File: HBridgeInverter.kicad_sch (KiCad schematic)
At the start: 27 parts, among them Q1 NMOS, Q2 NMOS, Q3 NMOS, Q4 NMOS, Q5 NMOS, Q6 NMOS, Q7 NPN, U1 LM358

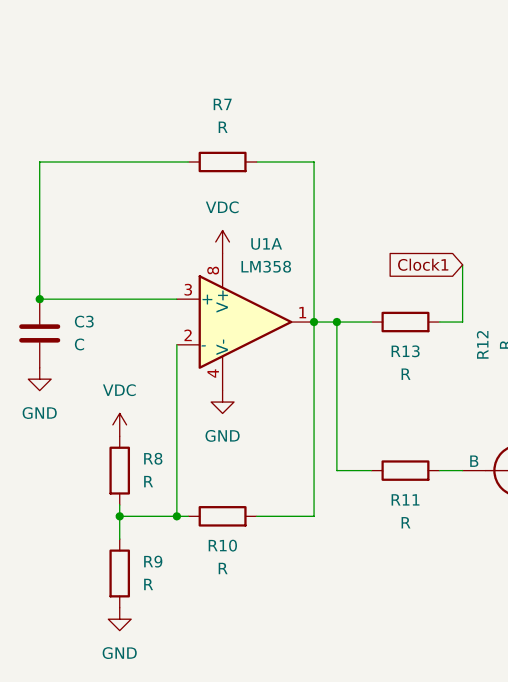
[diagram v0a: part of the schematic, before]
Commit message: whoops
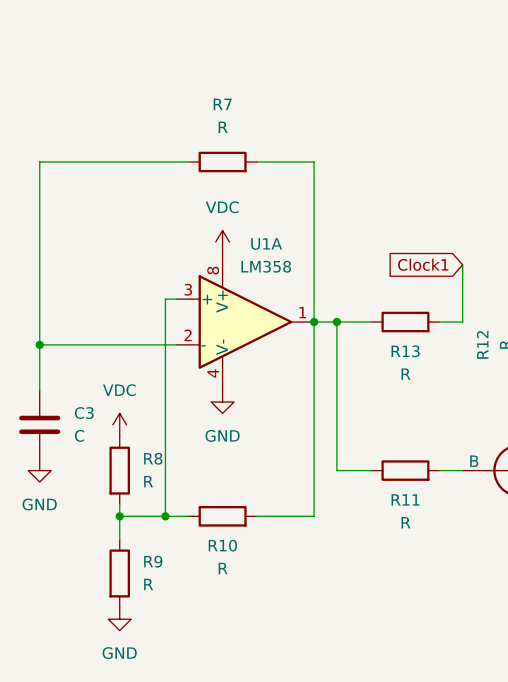
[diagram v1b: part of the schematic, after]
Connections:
- net at C3.1, R7.1: now also U1.2 (-); no longer U1.3 (+)
- net at R10.1, R8.2, R9.1: now also U1.3 (+); no longer U1.2 (-)
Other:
- moved on the sheet: C3
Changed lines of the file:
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@@
+	)
+	(junction
+		(at 48.26 106.68)
+		(diameter 0)
+		(color 0 0 0 0)
 	)
 	(junction
@@
 	)
 	(junction
-		(at 67.31 85.09)
+		(at 34.29 87.63)
 		(diameter 0)
 		(color 0 0 0 0)
 	)
 	(junction
-		(at 34.29 82.55)
+		(at 67.31 85.09)
 		(diameter 0)
 		(color 0 0 0 0)
@@
 	)
 	(junction
-		(at 49.53 106.68)
-		(diameter 0)
-		(color 0 0 0 0)
-	)
-	(junction
 		(at 190.5 81.28)
 		(diameter 0)
@@
 	(wire
 		(pts
+			(xy 48.26 106.68) (xy 50.8 106.68)
+		)
+		(stroke
+			(width 0)
+			(type default)
+		)
+	)
+	(wire
+		(pts
 			(xy 203.2 57.15) (xy 215.9 57.15)
 		)
@@
 	(wire
 		(pts
-			(xy 49.53 106.68) (xy 50.8 106.68)
-		)
-		(stroke
-			(width 0)
-			(type default)
-		)
-	)
-	(wire
-		(pts
 			(xy 215.9 73.66) (xy 215.9 95.25)
 		)
@@
 	(wire
 		(pts
+			(xy 49.53 82.55) (xy 48.26 82.55)
+		)
+		(stroke
+			(width 0)
+			(type default)
+		)
+	)
+	(wire
+		(pts
 			(xy 190.5 81.28) (xy 203.2 81.28)
 		)
@@
 	(wire
 		(pts
+			(xy 34.29 87.63) (xy 49.53 87.63)
+		)
+		(stroke
+			(width 0)
+			(type default)
+		)
+	)
+	(wire
+		(pts
 			(xy 64.77 67.31) (xy 64.77 85.09)
 		)
@@
 	(wire
 		(pts
+			(xy 34.29 87.63) (xy 34.29 92.71)
+		)
+		(stroke
+			(width 0)
+			(type default)
+		)
+	)
+	(wire
+		(pts
 			(xy 78.74 101.6) (xy 81.28 101.6)
 		)
@@
 	(wire
 		(pts
-			(xy 49.53 87.63) (xy 49.53 106.68)
-		)
-		(stroke
-			(width 0)
-			(type default)
-		)
-	)
-	(wire
-		(pts
 			(xy 152.4 95.25) (xy 152.4 101.6)
 		)
@@
 	(wire
 		(pts
-			(xy 34.29 67.31) (xy 34.29 82.55)
+			(xy 34.29 67.31) (xy 34.29 87.63)
 		)
 		(stroke
@@
 	(wire
 		(pts
-			(xy 34.29 82.55) (xy 49.53 82.55)
-		)
-		(stroke
-			(width 0)
-			(type default)
-		)
-	)
-	(wire
-		(pts
-			(xy 43.18 106.68) (xy 49.53 106.68)
+			(xy 43.18 106.68) (xy 48.26 106.68)
 		)
 		(stroke
@@
 		(pts
 			(xy 58.42 106.68) (xy 64.77 106.68)
+		)
+		(stroke
+			(width 0)
+			(type default)
+		)
+	)
+	(wire
+		(pts
+			(xy 48.26 82.55) (xy 48.26 106.68)
 		)
 		(stroke
@@
 	(symbol
 		(lib_id "Device:C")
-		(at 34.29 86.36 0)
+		(at 34.29 96.52 0)
 		(unit 1)
 		(exclude_from_sim no)
@@
 		(fields_autoplaced yes)
 		(property "Reference" "C3"
-			(at 38.1 85.0899 0)
+			(at 38.1 95.2499 0)
 			(effects
 				(font
@@
 		)
 		(property "Value" "C"
-			(at 38.1 87.6299 0)
+			(at 38.1 97.7899 0)
 			(effects
 				(font
@@
 		)
 		(property "Footprint" ""
-			(at 35.2552 90.17 0)
+			(at 35.2552 100.33 0)
 			(effects
 				(font
@@
 		)
 		(property "Datasheet" "~"
-			(at 34.29 86.36 0)
+			(at 34.29 96.52 0)
 			(effects
 				(font
@@
 		)
 		(property "Description" "Unpolarized capacitor"
-			(at 34.29 86.36 0)
+			(at 34.29 96.52 0)
 			(effects
 				(font
@@
 	(symbol
 		(lib_id "power:GND")
-		(at 34.29 90.17 0)
+		(at 34.29 100.33 0)
 		(unit 1)
 		(exclude_from_sim no)
@@
 		(fields_autoplaced yes)
 		(property "Reference" "#PWR013"
-			(at 34.29 96.52 0)
+			(at 34.29 106.68 0)
 			(effects
 				(font
@@
 		)
 		(property "Value" "GND"
-			(at 34.29 95.25 0)
+			(at 34.29 105.41 0)
 			(effects
 				(font
@@
 		)
 		(property "Footprint" ""
-			(at 34.29 90.17 0)
+			(at 34.29 100.33 0)
 			(effects
 				(font
@@
 		)
 		(property "Datasheet" ""
-			(at 34.29 90.17 0)
+			(at 34.29 100.33 0)
 			(effects
 				(font
@@
 		)
 		(property "Description" "Power symbol creates a global label with name \"GND\" , ground"
-			(at 34.29 90.17 0)
-			(effects
-				(font
+			(at 34.29 100.33 0)
+			(effects
+				(font
